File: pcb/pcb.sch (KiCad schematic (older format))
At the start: 318 parts, among them J1 USB_C_Receptacle_USB2.0, J2 ISP, SW1 SW_Push, SW10 SW_Push, SW11 SW_Push, SW12 SW_Push, SW13 SW_Push, SW14 SW_Push, SW15 SW_Push, SW16 SW_Push, SW18 SW_Push, SW19 SW_Push, SW2 SW_Push, SW20 SW_Push, SW21 SW_Push, SW22 SW_Push, SW23 SW_Push, SW24 SW_Push, SW25 SW_Push, SW26 SW_Push, SW27 SW_Push, SW28 SW_Push, SW29 SW_Push, SW3 SW_Push, SW30 SW_Push, SW31 SW_Push, SW32 SW_Push, SW33 SW_Push, SW34 SW_Push, SW35 SW_Push, SW36 SW_Push, SW37 SW_Push, SW38 SW_Push, SW39 SW_Push, SW4 SW_Push, SW40 SW_Push, SW41 SW_Push, SW42 SW_Push, SW43 SW_Push, SW44 SW_Push, SW45 SW_Push, SW46 SW_Push, SW47 SW_Push, SW48 SW_Push, SW49 SW_Push, SW5 SW_Push, SW50 SW_Push, SW51 SW_Push, SW52 SW_Push, SW53 SW_Push, SW54 SW_Push, SW55 SW_Push, SW56 SW_Push, SW57 SW_Push, SW58 SW_Push, SW59 SW_Push, SW6 SW_Push, SW60 SW_Push, SW61 SW_Push, SW62 SW_Push, SW63 SW_Push, SW64 SW_Push, SW65 SW_Push, SW66 SW_Push, SW67 SW_Push, SW68 SW_Push, SW69 SW_Push, SW7 SW_Push, SW70 SW_Push, SW71 SW_Push, SW72 SW_Push, SW73 SW_Push, SW74 SW_Push, SW75 SW_Push, SW76 SW_Push, SW77 SW_Push, SW78 SW_Push, SW79 SW_Push, SW8 SW_Push, SW80 SW_Push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

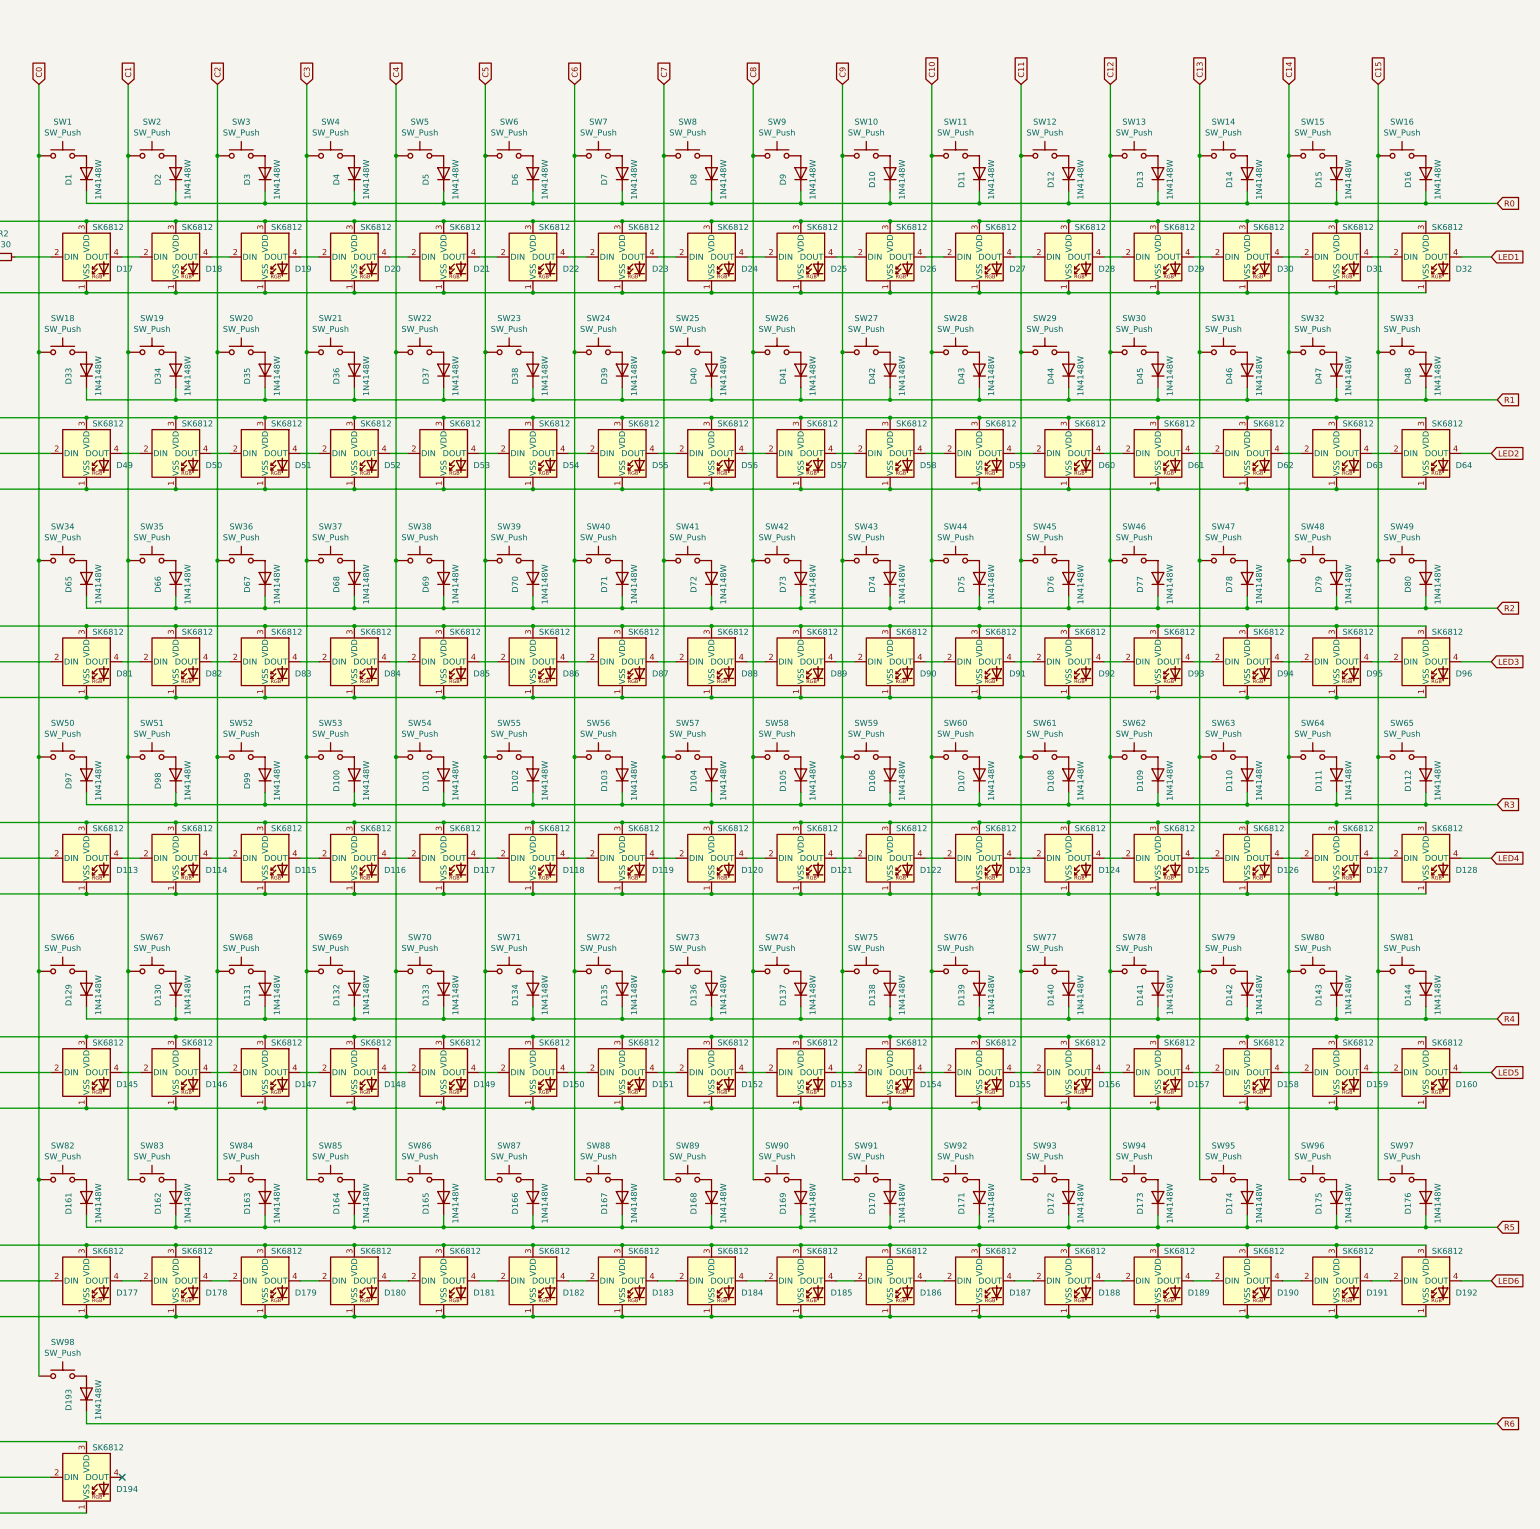
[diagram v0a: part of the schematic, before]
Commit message: working on pcb
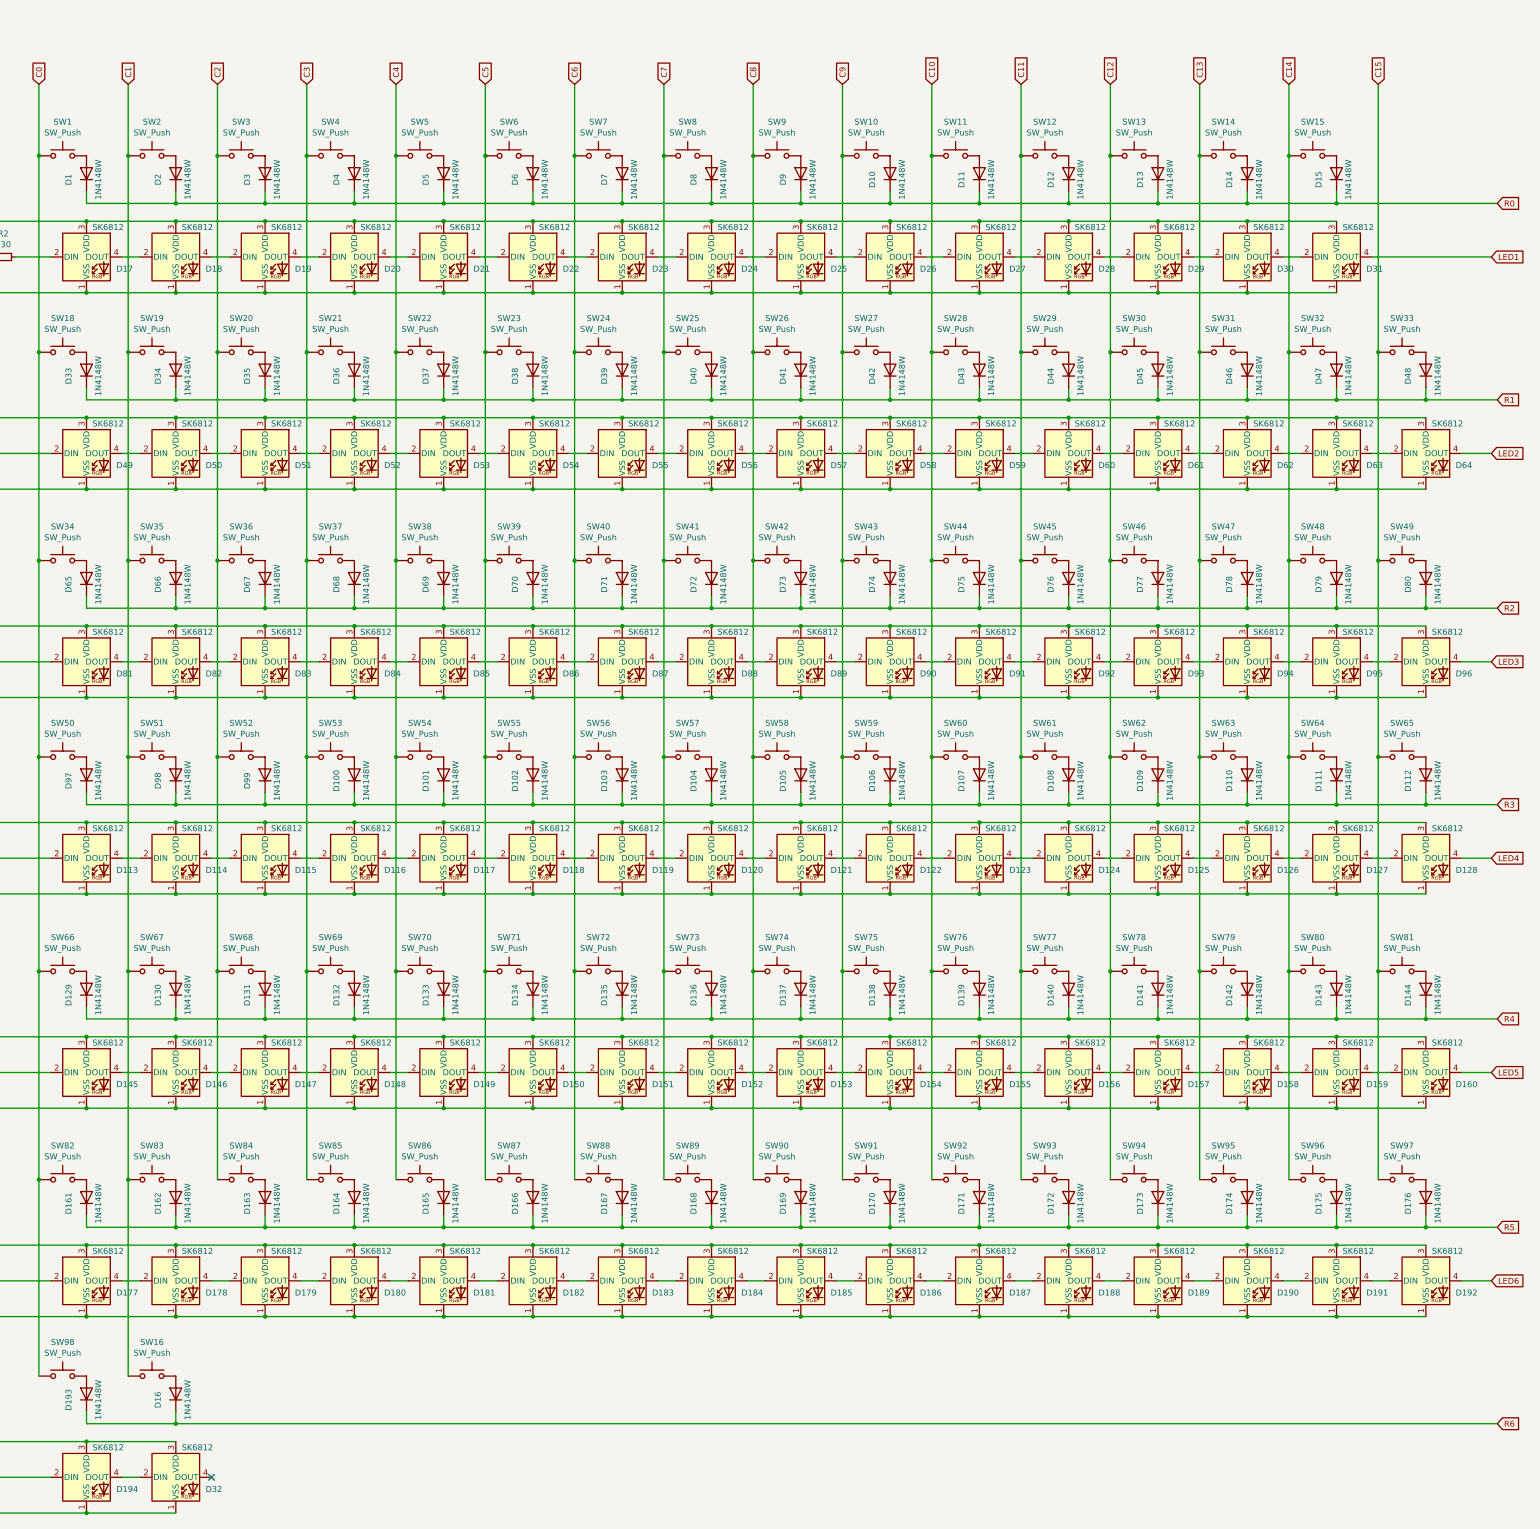
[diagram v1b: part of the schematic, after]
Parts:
- SW88: footprint Button_Switch_Keyboard:SW_Cherry_MX_1.00u_PCB -> Button_Switch_Keyboard:SW_Cherry_MX_1.50u_PCB
- SW94: footprint Button_Switch_Keyboard:SW_Cherry_MX_1.00u_PCB -> Button_Switch_Keyboard:SW_Cherry_MX_1.25u_PCB
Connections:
- net C1: now also SW16.1
- net C15: no longer SW16.1
- net LED1: now also D31.4 (DOUT); no longer D32.4 (DOUT)
- net R0: no longer D16.1 (K)
- net R6: now also D16.1 (K)
- net at D32.2 (DIN): now also D194.4 (DOUT); no longer D31.4 (DOUT)
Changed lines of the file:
@@
 	18150 3100 18900 3100
 Wire Wire Line
-	20400 3100 21150 3100
-Wire Wire Line
 	19650 3100 20400 3100
 Wire Wire Line
@@
 Text GLabel 21750 3100 2    50   Input ~ 0
 R0
-Wire Wire Line
-	21150 3100 21750 3100
-Connection ~ 21150 3100
-Connection ~ 20400 3100
 Connection ~ 18150 3100
 Connection ~ 17400 3100
@@
 Connection ~ 12150 3100
 Connection ~ 11400 3100
-Wire Wire Line
-	21150 3000 21150 3100
-$Comp
-L Switch:SW_Push SW16
-U 1 1 6406DE3F
-P 20950 2700
-F 0 "SW16" H 20950 2985 50  0000 C CNN
-F 1 "SW_Push" H 20950 2894 50  0000 C CNN
-F 2 "Button_Switch_Keyboard:SW_Cherry_MX_1.00u_PCB" H 20950 2900 50  0001 C CNN
-F 3 "~" H 20950 2900 50  0001 C CNN
-	1    20950 2700
-	1    0    0    -1
-$EndComp
 Text GLabel 20750 2100 1    50   Input ~ 0
 C15
-$Comp
-L Diode:1N4148W D16
-U 1 1 6406DE37
-P 21150 2850
-F 0 "D16" H 21100 3000 50  0000 C CNN
-F 1 "1N4148W" H 21100 2750 50  0000 C CNN
-F 2 "Diode_SMD:D_SOD-123" H 21150 2675 50  0001 C CNN
-F 3 "https://www.vishay.com/docs/85748/1n4148w.pdf" H 21150 2850 50  0001 C CNN
-	1    21150 2850
-	0    -1   -1   0
-$EndComp
 Wire Wire Line
 	20400 3000 20400 3100
@@
 Wire Wire Line
 	19950 3550 20100 3550
-Wire Wire Line
-	20700 3550 20850 3550
 $Comp
 L power:+5V #PWR06
@@
 Wire Wire Line
 	19650 3250 20400 3250
-Connection ~ 20400 3250
-Wire Wire Line
-	20400 3250 21150 3250
-Wire Wire Line
-	21150 3850 20400 3850
 Connection ~ 10650 3850
 Wire Wire Line
@@
 Wire Wire Line
 	19650 3850 18900 3850
-Connection ~ 20400 3850
 Wire Wire Line
 	20400 3850 19650 3850
@@
 F 0 "SW94" H 18700 11585 50  0000 C CNN
 F 1 "SW_Push" H 18700 11494 50  0000 C CNN
-F 2 "Button_Switch_Keyboard:SW_Cherry_MX_1.00u_PCB" H 18700 11500 50  0001 C CNN
+F 2 "Button_Switch_Keyboard:SW_Cherry_MX_1.25u_PCB" H 18700 11500 50  0001 C CNN
 F 3 "~" H 18700 11500 50  0001 C CNN
 	1    18700 11300
@@
 F 0 "SW88" H 14200 11585 50  0000 C CNN
 F 1 "SW_Push" H 14200 11494 50  0000 C CNN
-F 2 "Button_Switch_Keyboard:SW_Cherry_MX_1.00u_PCB" H 14200 11500 50  0001 C CNN
+F 2 "Button_Switch_Keyboard:SW_Cherry_MX_1.50u_PCB" H 14200 11500 50  0001 C CNN
 F 3 "~" H 14200 11500 50  0001 C CNN
 	1    14200 11300
@@
 	9600 12150 8950 12150
 Wire Wire Line
-	9900 13350 21750 13350
-NoConn ~ 10200 13800
-Wire Wire Line
 	8950 13800 9600 13800
 Wire Wire Line
@@
 Wire Wire Line
 	20000 9550 20000 11300
-Wire Wire Line
-	20750 2100 20750 2700
-Connection ~ 20750 2700
-Wire Wire Line
-	20750 2700 20750 4350
 Connection ~ 20750 4350
 Wire Wire Line
@@
 	1    0    0    -1
 $EndComp
-$Comp
-L LED:SK6812 D32
-U 1 1 6484D498
-P 21150 3550
-F 0 "D32" H 21400 3450 50  0000 L CNN
-F 1 "SK6812" H 21200 3800 50  0000 L CNN
-F 2 "LED_SMD:LED_SK6812_PLCC4_5.0x5.0mm_P3.2mm" H 21200 3250 50  0001 L TNN
-F 3 "https://cdn-shop.adafruit.com/product-files/1138/SK6812+LED+datasheet+.pdf" H 21250 3175 50  0001 L TNN
-	1    21150 3550
-	1    0    0    -1
-$EndComp
 Text GLabel 8950 12150 0    50   Input ~ 0
 LED5
@@
 Text GLabel 21700 5200 2    50   Input ~ 0
 LED2
-Wire Wire Line
-	21450 3550 21700 3550
 Text GLabel 21700 3550 2    50   Input ~ 0
 LED1
@@
 	0    -1   -1   0
 $EndComp
+Wire Wire Line
+	20750 2100 20750 4350
+Wire Wire Line
+	21750 3100 20400 3100
+Connection ~ 20400 3100
+Wire Wire Line
+	21700 3550 20700 3550
+Wire Wire Line
+	10650 13250 10650 13350
+$Comp
+L Switch:SW_Push SW16
+U 1 1 644B1697
+P 10450 12950
+F 0 "SW16" H 10450 13235 50  0000 C CNN
+F 1 "SW_Push" H 10450 13144 50  0000 C CNN
+F 2 "Button_Switch_Keyboard:SW_Cherry_MX_1.00u_PCB" H 10450 13150 50  0001 C CNN
+F 3 "~" H 10450 13150 50  0001 C CNN
+	1    10450 12950
+	1    0    0    -1
+$EndComp
+$Comp
+L Diode:1N4148W D16
+U 1 1 644B169D
+P 10650 13100
+F 0 "D16" H 10600 13250 50  0000 C CNN
+F 1 "1N4148W" H 10600 13000 50  0000 C CNN
+F 2 "Diode_SMD:D_SOD-123" H 10650 12925 50  0001 C CNN
+F 3 "https://www.vishay.com/docs/85748/1n4148w.pdf" H 10650 13100 50  0001 C CNN
+	1    10650 13100
+	0    -1   -1   0
+$EndComp
+$Comp
+L LED:SK6812 D32
+U 1 1 644B16A6
+P 10650 13800
+F 0 "D32" H 10900 13700 50  0000 L CNN
+F 1 "SK6812" H 10700 14050 50  0000 L CNN
+F 2 "LED_SMD:LED_SK6812_PLCC4_5.0x5.0mm_P3.2mm" H 10700 13500 50  0001 L TNN
+F 3 "https://cdn-shop.adafruit.com/product-files/1138/SK6812+LED+datasheet+.pdf" H 10750 13425 50  0001 L TNN
+	1    10650 13800
+	1    0    0    -1
+$EndComp
+Wire Wire Line
+	10250 12950 10250 11300
+Connection ~ 10250 11300
+Wire Wire Line
+	9900 13350 10650 13350
+Connection ~ 10650 13350
+Wire Wire Line
+	10650 13350 21750 13350
+Wire Wire Line
+	9900 13500 10650 13500
+Connection ~ 9900 13500
+Wire Wire Line
+	9900 14100 10650 14100
+Connection ~ 9900 14100
+Wire Wire Line
+	10200 13800 10350 13800
+NoConn ~ 10950 13800
 $EndSCHEMATC
